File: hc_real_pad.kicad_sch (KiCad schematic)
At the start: 55 parts, among them J1 OLED_DISPLAY, SW1 SW_Push_45deg, SW10 SW_Push_45deg, SW11 SW_Push_45deg, SW12 SW_Push_45deg, SW13 SW_Push_45deg, SW14 SW_Push_45deg, SW15 SW_Push_45deg, SW16 SW_Push_45deg, SW17 RotaryEncoder_Switch, SW18 RotaryEncoder_Switch, SW2 SW_Push_45deg, SW3 SW_Push_45deg, SW4 SW_Push_45deg, SW5 SW_Push_45deg, SW6 SW_Push_45deg, SW7 SW_Push_45deg, SW8 SW_Push_45deg, SW9 SW_Push_45deg, U1 MOUDLE-SEEEDUINO-XIAO, U3 MCP23017_SP

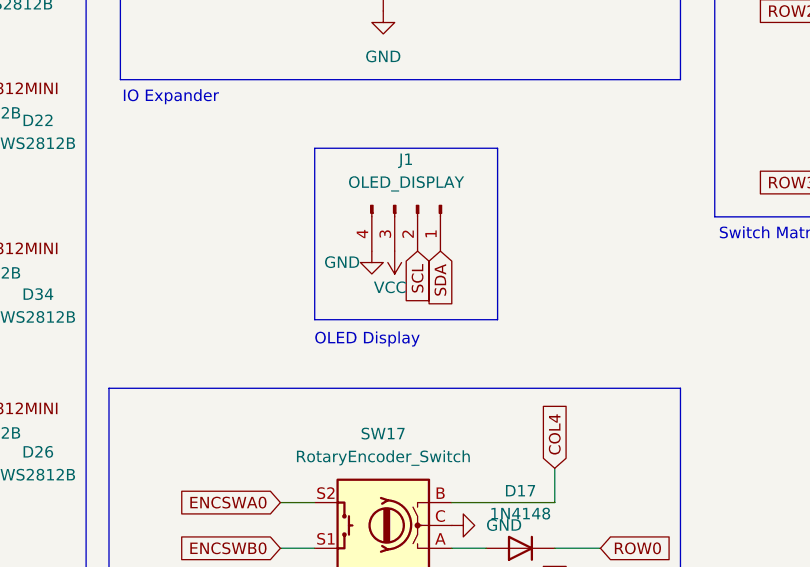
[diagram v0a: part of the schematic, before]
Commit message: finished making the pcb
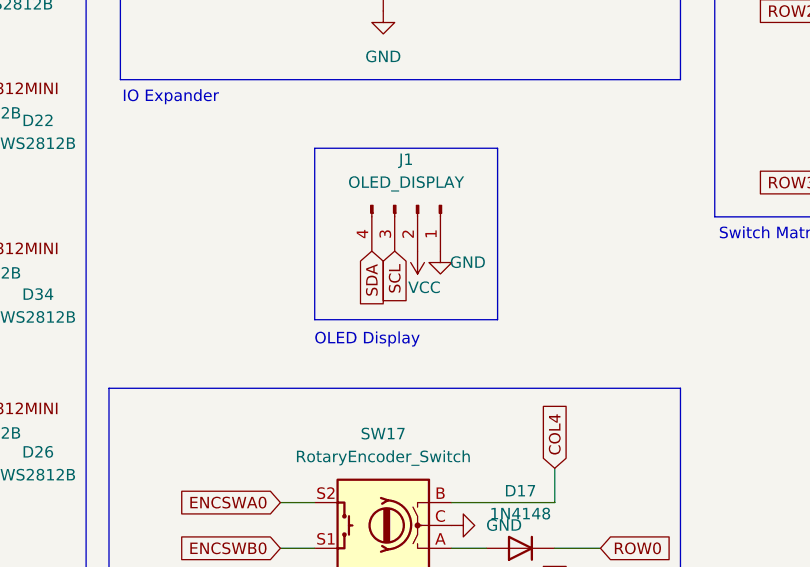
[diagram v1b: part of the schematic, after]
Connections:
- net GND: now also J1.1 (Pin_1); no longer J1.4 (Pin_4)
- net SCL: now also J1.3 (Pin_3); no longer J1.2 (Pin_2)
- net SDA: now also J1.4 (Pin_4); no longer J1.1 (Pin_1)
- net VCC: now also J1.2 (Pin_2); no longer J1.3 (Pin_3)
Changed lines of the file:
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@@
 	(global_label "SDA"
 		(shape input)
-		(at 144.78 106.68 270)
+		(at 137.16 106.68 270)
 		(fields_autoplaced yes)
 		(effects
@@
 		)
 		(property "Intersheetrefs" "${INTERSHEET_REFS}"
-			(at 144.78 113.2333 90)
+			(at 137.16 113.2333 90)
 			(effects
 				(font
@@
 	(global_label "SCL"
 		(shape input)
-		(at 142.24 106.68 270)
+		(at 139.7 106.68 270)
 		(fields_autoplaced yes)
 		(effects
@@
 		)
 		(property "Intersheetrefs" "${INTERSHEET_REFS}"
-			(at 142.24 113.1728 90)
+			(at 139.7 113.1728 90)
 			(effects
 				(font
@@
 	(symbol
 		(lib_id "power:GND")
-		(at 137.16 106.68 0)
+		(at 144.78 106.68 0)
 		(unit 1)
 		(exclude_from_sim no)
@@
 		(dnp no)
 		(property "Reference" "#PWR09"
-			(at 137.16 113.03 0)
+			(at 144.78 113.03 0)
 			(effects
 				(font
@@
 		)
 		(property "Value" "GND"
-			(at 133.858 107.95 0)
+			(at 147.828 107.95 0)
 			(effects
 				(font
@@
 		)
 		(property "Footprint" ""
-			(at 137.16 106.68 0)
+			(at 144.78 106.68 0)
 			(effects
 				(font
@@
 		)
 		(property "Datasheet" ""
-			(at 137.16 106.68 0)
+			(at 144.78 106.68 0)
 			(effects
 				(font
@@
 		)
 		(property "Description" "Power symbol creates a global label with name \"GND\" , ground"
-			(at 137.16 106.68 0)
+			(at 144.78 106.68 0)
 			(effects
 				(font
@@
 	(symbol
 		(lib_id "power:VCC")
-		(at 139.7 106.68 180)
+		(at 142.24 106.68 180)
 		(unit 1)
 		(exclude_from_sim no)
@@
 		(dnp no)
 		(property "Reference" "#PWR08"
-			(at 139.7 102.87 0)
+			(at 142.24 102.87 0)
 			(effects
 				(font
@@
 		)
 		(property "Value" "VCC"
-			(at 139.192 110.744 0)
+			(at 143.002 110.744 0)
 			(effects
 				(font
@@
 		)
 		(property "Footprint" ""
-			(at 139.7 106.68 0)
+			(at 142.24 106.68 0)
 			(effects
 				(font
@@
 		)
 		(property "Datasheet" ""
-			(at 139.7 106.68 0)
+			(at 142.24 106.68 0)
 			(effects
 				(font
@@
 		)
 		(property "Description" "Power symbol creates a global label with name \"VCC\""
-			(at 139.7 106.68 0)
+			(at 142.24 106.68 0)
 			(effects
 				(font
